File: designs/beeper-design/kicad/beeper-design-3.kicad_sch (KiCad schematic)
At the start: 30 parts, among them U12 DRV2605YZFR, U13 CSD75207W15, U3 BQ51003YFPR

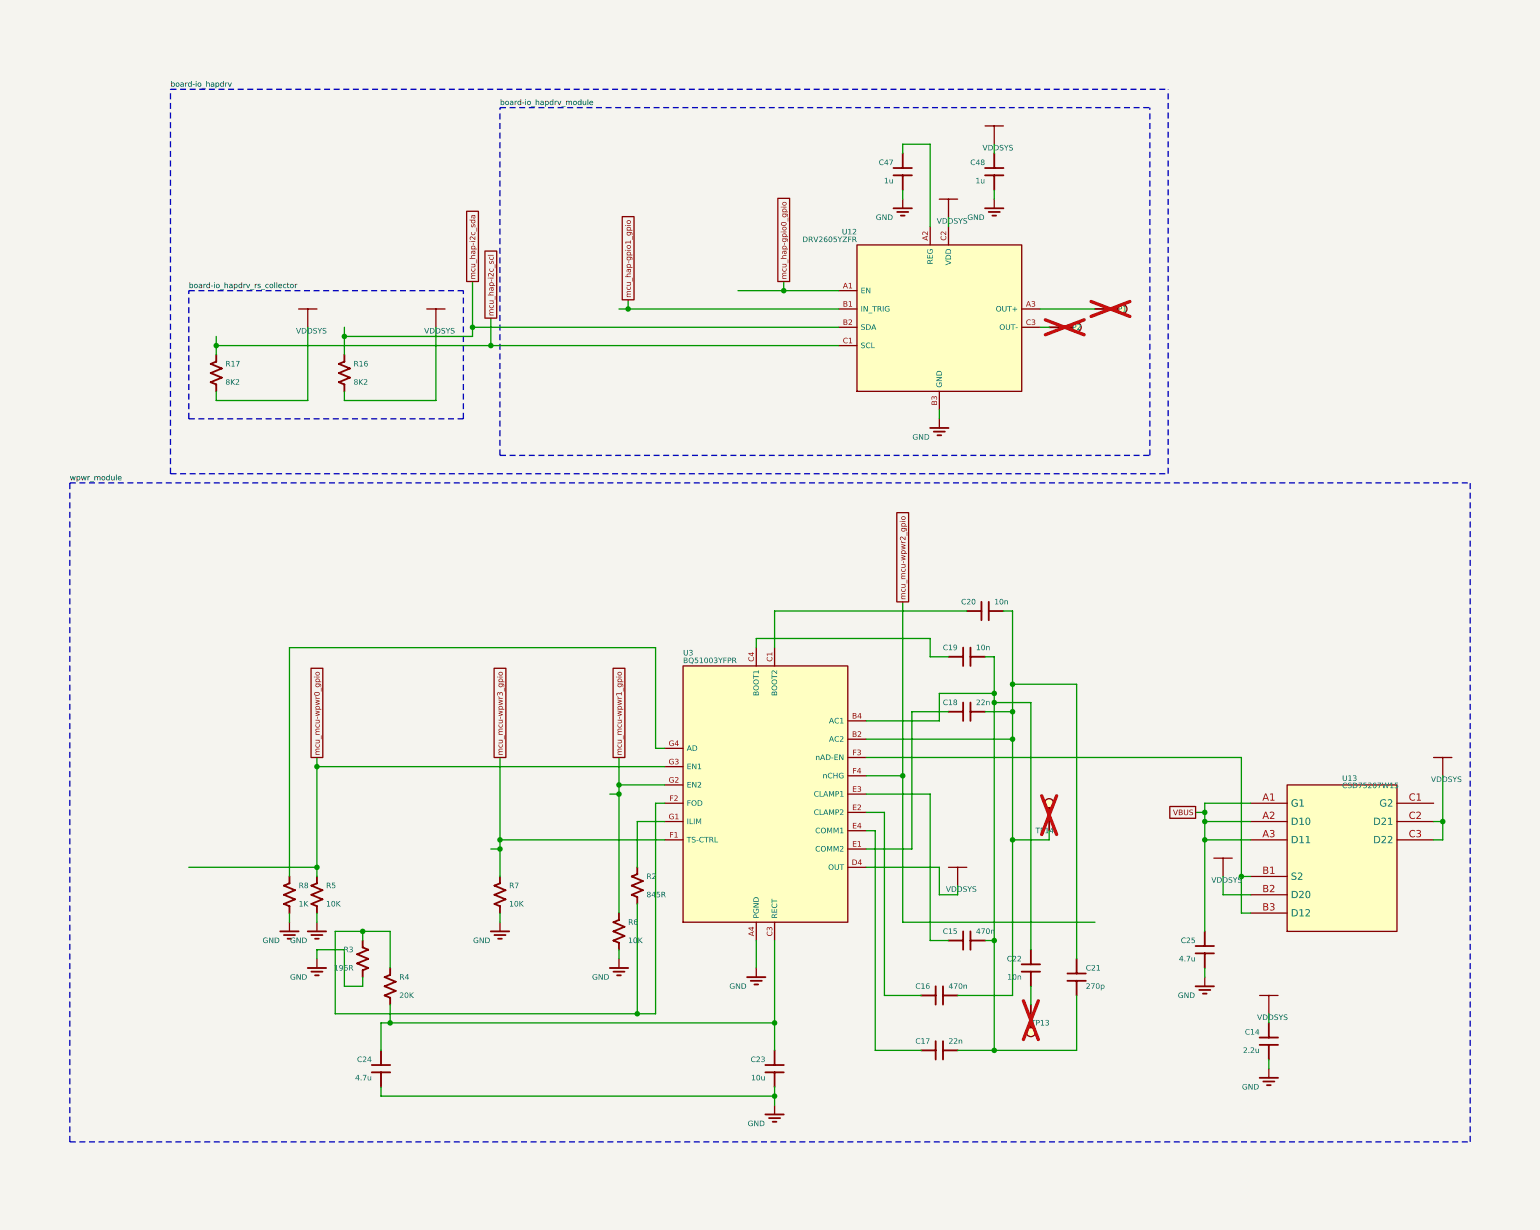
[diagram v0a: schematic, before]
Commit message: kicad exported data
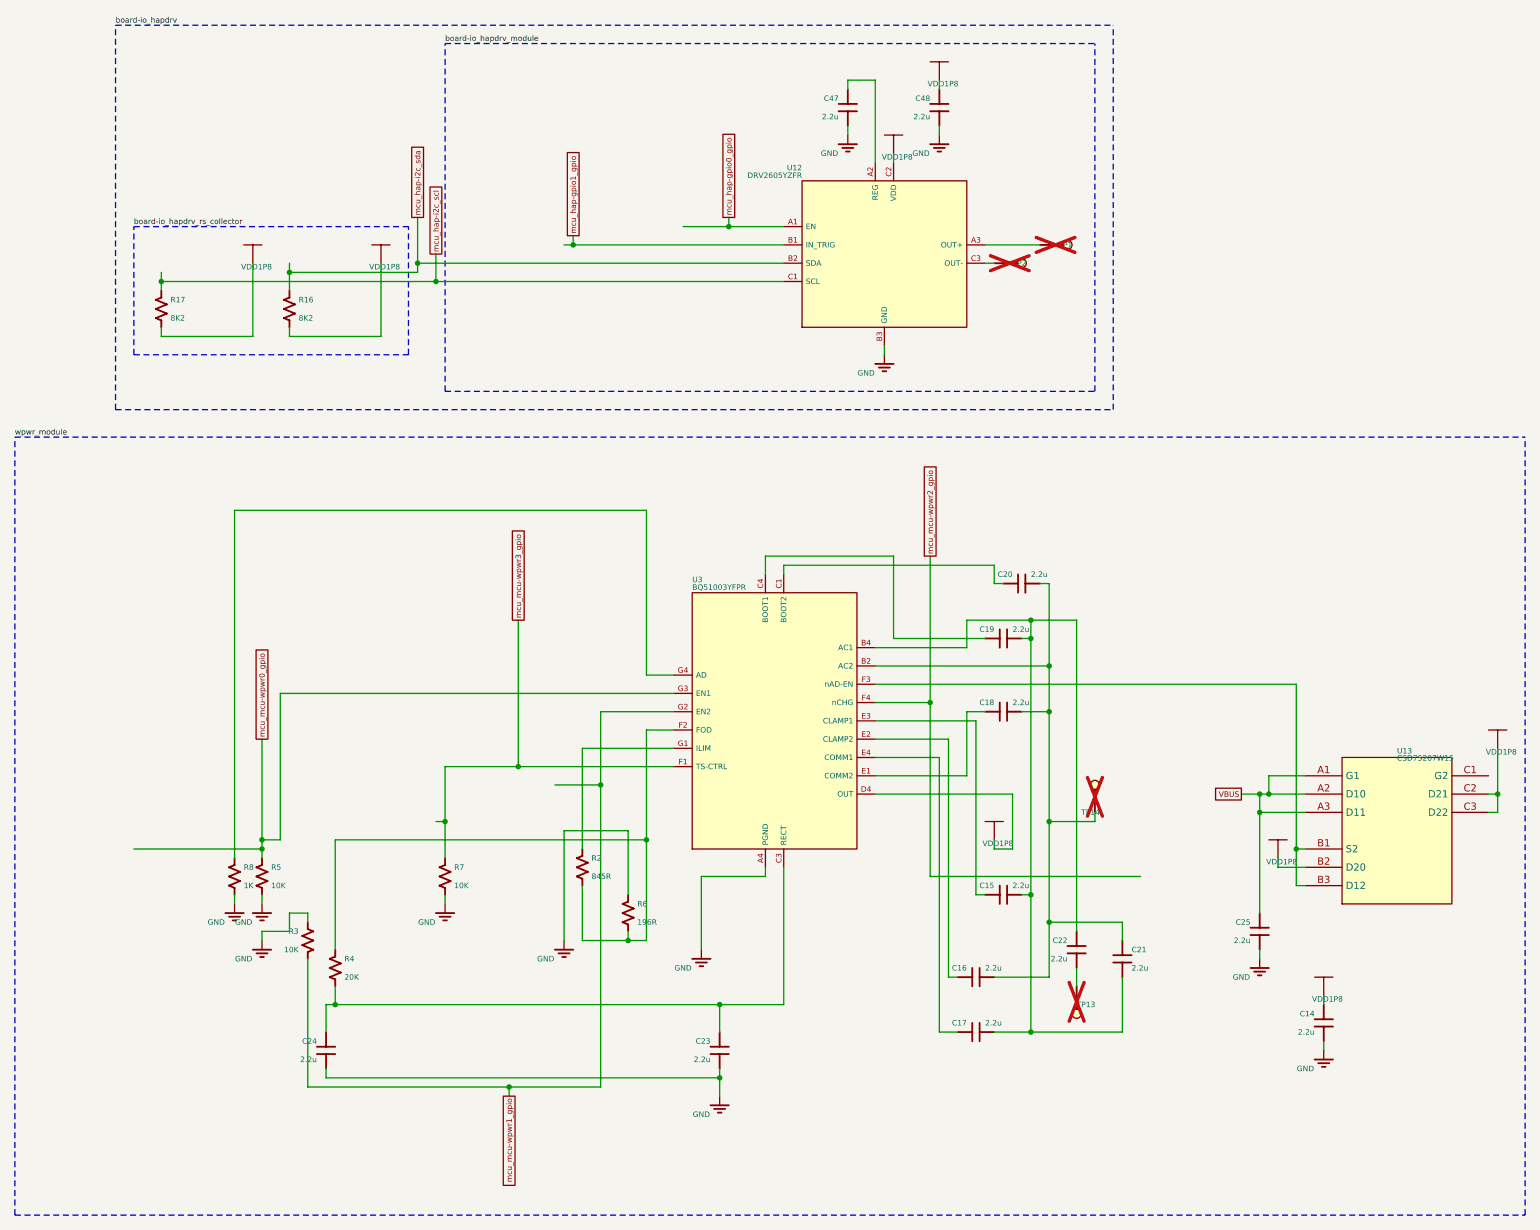
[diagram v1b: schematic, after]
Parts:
- removed C14: 2.2u, beeper-design:Pkg0201_25, symbol my_capacitor_7
- removed C15: 470n, beeper-design:Pkg0201_21, symbol my_capacitor_5
- removed C16: 470n, beeper-design:Pkg0201_31, symbol my_capacitor_10
- removed C17: 22n, beeper-design:Pkg0201_45, symbol my_capacitor_18
- removed C18: 22n, beeper-design:Pkg0201_9, symbol my_capacitor_2
- removed C19: 10n, beeper-design:Pkg0201_18, symbol my_capacitor_4
- removed C20: 10n, beeper-design:Pkg0201_30, symbol my_capacitor_9
- removed C21: 270p, beeper-design:Pkg0201_43, symbol my_capacitor_16
- removed C22: 10n, beeper-design:Pkg0201_7, symbol my_capacitor
- removed C23: 10u, beeper-design:Pkg0402_2, symbol C105225_2
- removed C24: 4.7u, beeper-design:Pkg0402_6, symbol C23733_1
- removed C25: 4.7u, beeper-design:Pkg0402_4, symbol C23733
- removed C47: 1u, beeper-design:Pkg0201_40, symbol C76935_11
- removed C48: 1u, beeper-design:Pkg0201_6, symbol C76935_2
- removed R16, R17: 8K2, beeper-design:Pkg0201_20, symbol my_resistor_6
- removed R2: 845R, beeper-design:Pkg0201_36, symbol my_resistor_10
- removed R3: 196R, beeper-design:Pkg0201_2, symbol C138167
- removed R4: 20K, beeper-design:Pkg0201_12, symbol my_resistor_3
- removed R5: 10K, beeper-design:Pkg0201_22, symbol my_resistor_7
- removed R6: 10K, beeper-design:Pkg0201_34, symbol my_resistor_9
- removed R7: 10K, beeper-design:Pkg0201, symbol my_resistor_12
- removed R8: 1K, beeper-design:Pkg0201_11, symbol my_resistor_2
- added C14: 2.2u, beeper-design:Pkg0201_18, symbol C335106_9
- added C15: 2.2u, beeper-design:Pkg0201_11, symbol C335106_5
- added C16: 2.2u, beeper-design:Pkg0201_27, symbol C335106_17
- added C17: 2.2u, beeper-design:Pkg0201_40, symbol C335106_26
- added C18: 2.2u, beeper-design:Pkg0201_53, symbol C335106_35
- added C19: 2.2u, beeper-design:Pkg0201_10, symbol C335106_4
- added C20: 2.2u, beeper-design:Pkg0201_26, symbol C335106_16
- added C21: 2.2u, beeper-design:Pkg0201_39, symbol C335106_25
- added C22: 2.2u, beeper-design:Pkg0201_52, symbol C335106_34
- added C23: 2.2u, beeper-design:Pkg0201_9, symbol C335106_3
- added C24: 2.2u, beeper-design:Pkg0201_23, symbol C335106_13
- added C25: 2.2u, beeper-design:Pkg0201_16, symbol C335106_7
- added C47: 2.2u, beeper-design:Pkg0201_35, symbol C335106_23
- added C48: 2.2u, beeper-design:Pkg0201_47, symbol C335106_29
- added R16, R17: 8K2, beeper-design:Pkg0201_8, symbol my_resistor_3
- added R2: 845R, beeper-design:Pkg0201_32, symbol my_resistor_7
- added R3: 10K, beeper-design:Pkg0201_30, symbol my_resistor_6
- added R4: 20K, beeper-design:Pkg0201_2, symbol my_resistor
- added R5: 10K, beeper-design:Pkg0201_15, symbol my_resistor_4
- added R6: 196R, beeper-design:Pkg0201_45, symbol C138167
- added R7: 10K, beeper-design:Pkg0201_41, symbol my_resistor_9
- added R8: 1K, beeper-design:Pkg0201_54, symbol my_resistor_12
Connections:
- net GND: now also C14.1, C23.1, C24.1, C25.1, C47.1, C48.1, R3.2, R5.2, R6.2, R7.2, R8.2
- net VBUS: now also C25.2
- net mcu_hap-i2c_scl: now also R17.1
- net mcu_hap-i2c_sda: now also R16.1
- net mcu_mcu-wpwr0_gpio: now also R5.1
- net mcu_mcu-wpwr1_gpio: now also R3.1
- net mcu_mcu-wpwr3_gpio: now also R7.1
- net at TP14.p, U3.B1 (AC2), U3.B2 (AC2): now also C16.1, C18.1, C20.1, C21.1
- net at U3.E2 (CLAMP2): now also C16.2
- net at U12.A2 (REG): now also C47.2
- net at U3.G4 (AD): now also R8.1
- net at U3.C2 (RECT), U3.C3 (RECT): now also C23.2, C24.2, R4.2
- net at TP13.p: now also C22.1
- net at U3.B3 (AC1), U3.B4 (AC1): now also C15.1, C17.1, C19.1, C21.2, C22.2
- net at U3.F2 (FOD): now also R2.2, R4.1, R6.1
- net at U3.G1 (ILIM): now also R2.1
- net at U3.C4 (BOOT1): now also C19.2
- net at U3.E3 (CLAMP1): now also C15.2
- net at U3.C1 (BOOT2): now also C20.2
- net at U3.E4 (COMM1): now also C17.2
- net at U3.E1 (COMM2): now also C18.2
- net VDDSYS renamed VDD1P8
- net VDD1P8: now also C14.2, C48.2, R16.2, R17.2
